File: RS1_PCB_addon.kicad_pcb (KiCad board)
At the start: 2 copper layers, 45.6 x 35.6 mm, 31 parts, among them J1 Conn_01x02, J10 Conn_01x02, J2 SJ-3523-SMT-TR, J3 Conn_01x10_Socket, J5 Conn_01x05, J9 Conn_01x02, P2 S2B-PH-SM4-TB, U1 TPS2113ADRBR, U11 LTV-217-B-G, U12 LTV-217-B-G, U3 Adress 0x21 (cutable), U4 MCP23017_ML, U5 MAX17048G_T10

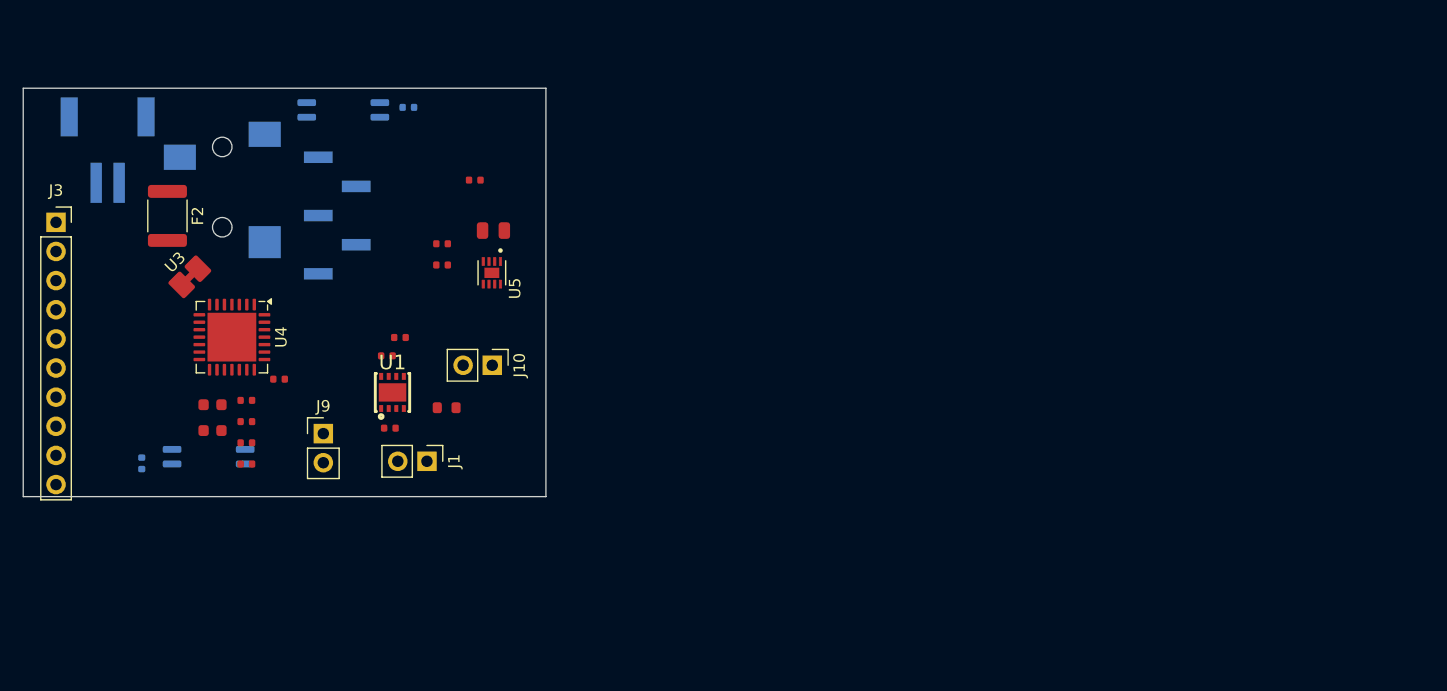
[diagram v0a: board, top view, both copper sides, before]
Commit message: change edgecut
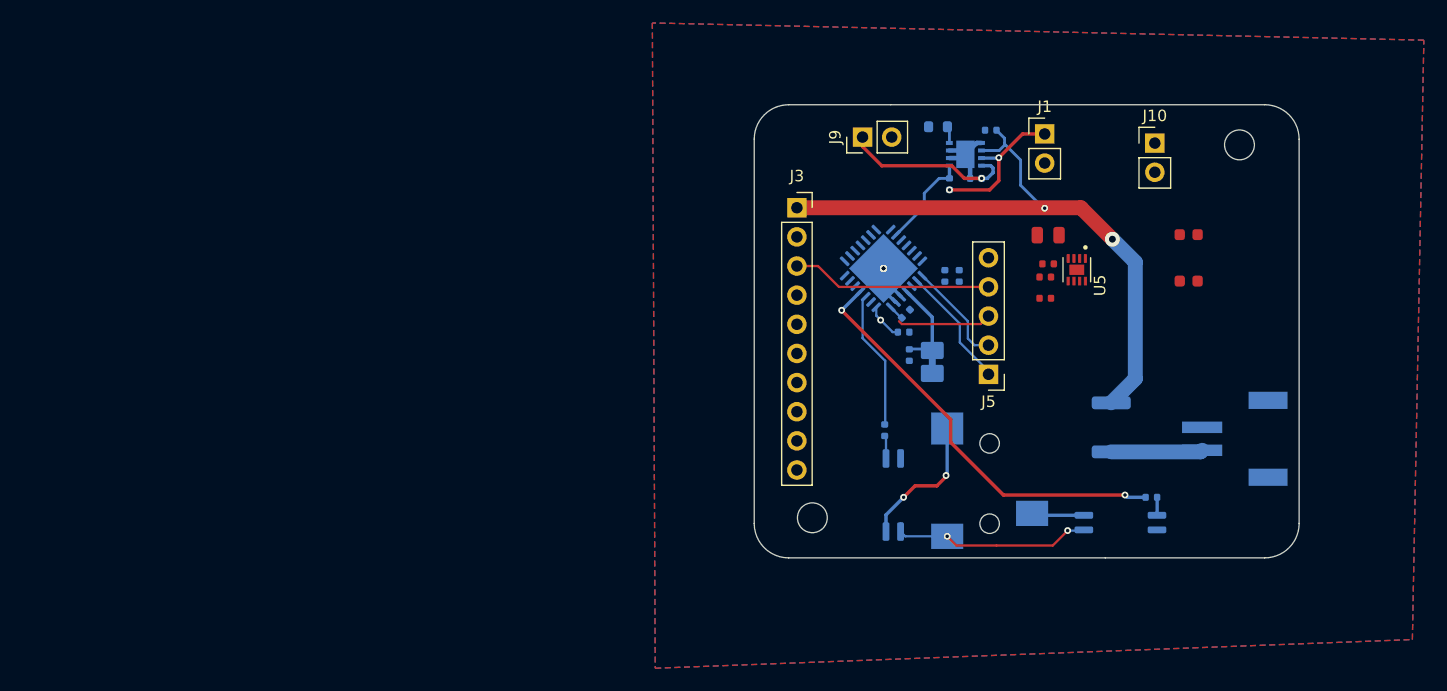
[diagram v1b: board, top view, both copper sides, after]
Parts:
- C1, C2, F2, R14, R15, R16, R17, R18, R2, R5, U1, U3, U4: moved to B.Cu
- J5: footprint Connector_PinHeader_2.54mm:PinHeader_1x05_P2.54mm_Vertical_SMD_Pin1Right -> Connector_PinHeader_2.54mm:PinHeader_1x05_P2.54mm_Vertical; moved to F.Cu
- moved P2 98.0 mm to (128.4, 66.5), turned to 90 degrees
- moved R20 88.1 mm to (124.0, 71.6), turned to 0 degrees
- moved C10 86.4 mm to (127.2, 48.7)
- moved C11 86.1 mm to (127.2, 52.8), turned to 180 degrees
- moved F2 84.3 mm to (120.5, 65.5), turned to 90 degrees
- moved U12 79.7 mm to (121.3, 73.8), turned to 180 degrees
- moved J2 74.5 mm to (109.9, 73.9), turned to 90 degrees
- moved U3 65.1 mm to (104.9, 59.8), turned to -90 degrees
- moved J3 64.6 mm to (93.1, 46.4)
- moved R15 63.4 mm to (107.2, 52.3), turned to -90 degrees
- moved R14 61.8 mm to (106.0, 52.3), turned to -90 degrees
- moved J1 60.9 mm to (114.7, 39.9), turned to 0 degrees
- moved J10 60.9 mm to (124.3, 40.7), turned to 0 degrees
- moved R17 59.0 mm to (102.6, 55.6), turned to 45 degrees
- moved U11 58.5 mm to (101.5, 71.4), turned to -90 degrees
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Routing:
- net /VBAT: track 0.00 -> 55.5 mm, vias 0 -> 2
- net /Op_2: track 0.00 -> 36.7 mm, vias 0 -> 2
- net Net-(J2-Pad1): track 0.00 -> 18.6 mm, vias 0 -> 2
- net /SERVO_PWM: track 0.00 -> 17.5 mm
- net +5V: track 0.00 -> 15.1 mm, vias 0 -> 1
- net GND: track 0.00 -> 13.7 mm, vias 0 -> 4
- net /VSYS: track 0.00 -> 13.0 mm, vias 0 -> 2
- net Net-(J2-Pad2): track 0.00 -> 12.3 mm, vias 0 -> 2
- net /Op_1: track 0.00 -> 12.1 mm
- net /INT_B: track 0.00 -> 11.1 mm, vias 0 -> 1
- net /SDA: track 0.00 -> 10.7 mm
- net /SCL: track 0.00 -> 9.16 mm
- net /STAT_Power_Path: track 0.00 -> 8.50 mm
- net Net-(F2-Pad1): track 0.00 -> 7.98 mm
- net Net-(U4-A0): track 0.00 -> 7.93 mm
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- added copper zone on B.Cu, net GND
- added copper zone on F.Cu, net GND
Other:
- board size 45.6 x 35.6 mm -> 47.5 x 39.5 mm
